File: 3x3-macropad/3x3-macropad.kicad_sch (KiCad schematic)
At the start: 38 parts, among them SW1 SW_Push, SW2 RotaryEncoder_Switch, U1 ATmega32U4-A, Y1 16MHz

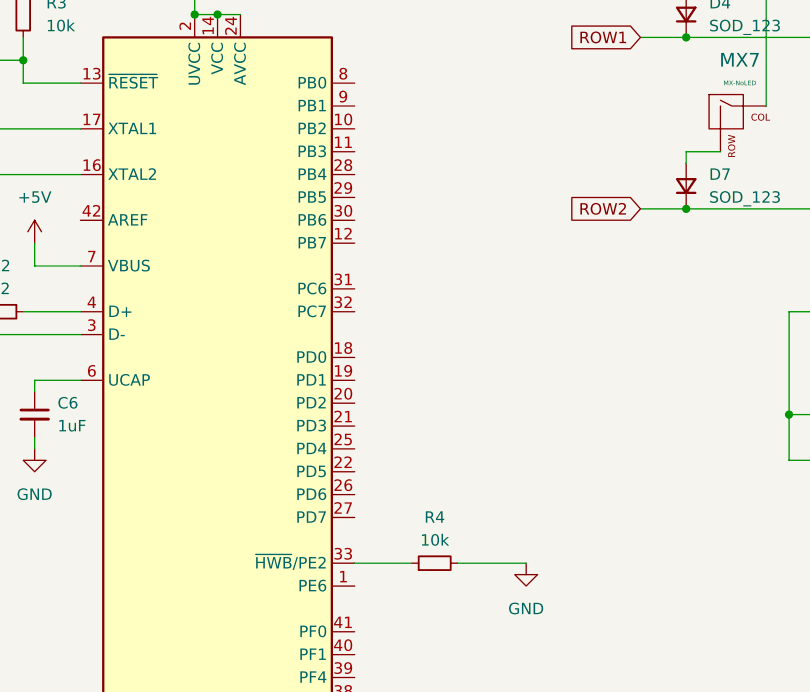
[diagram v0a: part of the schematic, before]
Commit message: first attempt routing 3x3
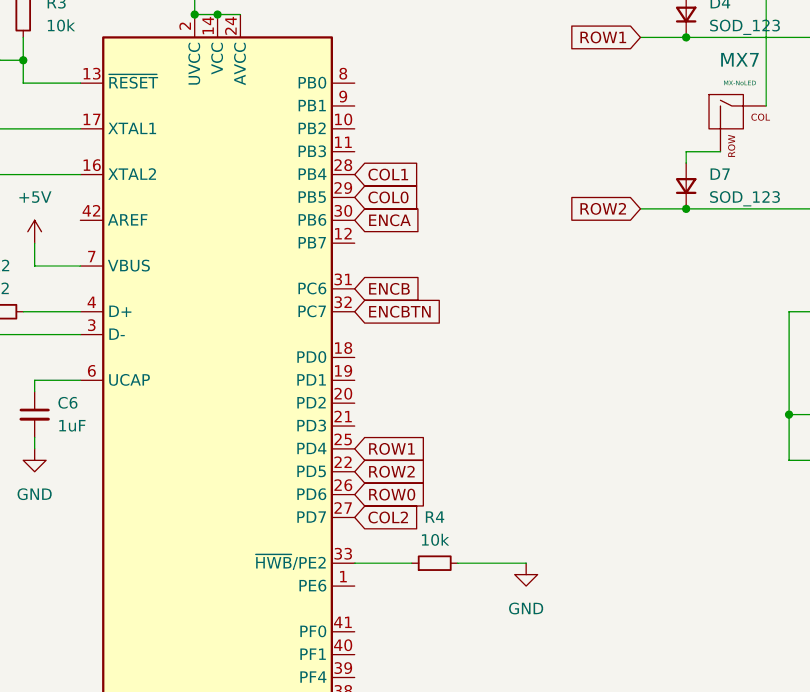
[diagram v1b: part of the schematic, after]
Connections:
- net COL0: now also U1.29 (PB5)
- net COL1: now also U1.28 (PB4)
- net COL2: now also U1.27 (PD7)
- net ENCA: now also U1.30 (PB6)
- net ENCB: now also U1.31 (PC6)
- net ENCBTN: now also U1.32 (PC7)
- net ROW0: now also U1.26 (PD6)
- net ROW1: now also U1.25 (PD4)
- net ROW2: now also U1.22 (PD5)
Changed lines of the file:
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@@
+    )
+  )
+  (global_label "ROW0" (shape input) (at 151.13 114.3 0) (fields_autoplaced)
+    (effects (font (size 1.27 1.27)) (justify left))
+    (property "Intersheetrefs" "${INTERSHEET_REFS}" (at 159.2972 114.3 0)
+      (effects (font (size 1.27 1.27)) (justify left) hide)
     )
   )
@@
     (effects (font (size 1.27 1.27)) (justify left))
     (property "Intersheetrefs" "${INTERSHEET_REFS}" (at 227.33 16.3861 90)
+      (effects (font (size 1.27 1.27)) (justify left) hide)
+    )
+  )
+  (global_label "COL1" (shape input) (at 151.13 78.74 0) (fields_autoplaced)
+    (effects (font (size 1.27 1.27)) (justify left))
+    (property "Intersheetrefs" "${INTERSHEET_REFS}" (at 158.8739 78.74 0)
+      (effects (font (size 1.27 1.27)) (justify left) hide)
+    )
+  )
+  (global_label "ENCBTN" (shape input) (at 151.13 93.98 0) (fields_autoplaced)
+    (effects (font (size 1.27 1.27)) (justify left))
+    (property "Intersheetrefs" "${INTERSHEET_REFS}" (at 161.3534 93.98 0)
+      (effects (font (size 1.27 1.27)) (justify left) hide)
+    )
+  )
+  (global_label "COL2" (shape input) (at 151.13 116.84 0) (fields_autoplaced)
+    (effects (font (size 1.27 1.27)) (justify left))
+    (property "Intersheetrefs" "${INTERSHEET_REFS}" (at 158.8739 116.84 0)
+      (effects (font (size 1.27 1.27)) (justify left) hide)
+    )
+  )
+  (global_label "COL0" (shape input) (at 151.13 81.28 0) (fields_autoplaced)
+    (effects (font (size 1.27 1.27)) (justify left))
+    (property "Intersheetrefs" "${INTERSHEET_REFS}" (at 158.8739 81.28 0)
+      (effects (font (size 1.27 1.27)) (justify left) hide)
+    )
+  )
+  (global_label "ENCA" (shape input) (at 151.13 83.82 0) (fields_autoplaced)
+    (effects (font (size 1.27 1.27)) (justify left))
+    (property "Intersheetrefs" "${INTERSHEET_REFS}" (at 158.8739 83.82 0)
       (effects (font (size 1.27 1.27)) (justify left) hide)
     )
@@
     (property "Intersheetrefs" "${INTERSHEET_REFS}" (at 212.09 128.3939 90)
       (effects (font (size 1.27 1.27)) (justify right) hide)
+    )
+  )
+  (global_label "ROW2" (shape input) (at 151.13 111.76 0) (fields_autoplaced)
+    (effects (font (size 1.27 1.27)) (justify left))
+    (property "Intersheetrefs" "${INTERSHEET_REFS}" (at 159.2972 111.76 0)
+      (effects (font (size 1.27 1.27)) (justify left) hide)
     )
   )
@@
     (effects (font (size 1.27 1.27)) (justify left))
     (property "Intersheetrefs" "${INTERSHEET_REFS}" (at 196.85 16.3861 90)
+      (effects (font (size 1.27 1.27)) (justify left) hide)
+    )
+  )
+  (global_label "ENCB" (shape input) (at 151.13 91.44 0) (fields_autoplaced)
+    (effects (font (size 1.27 1.27)) (justify left))
+    (property "Intersheetrefs" "${INTERSHEET_REFS}" (at 159.0553 91.44 0)
       (effects (font (size 1.27 1.27)) (justify left) hide)
     )
@@
     )
   )
+  (global_label "ROW1" (shape input) (at 151.13 109.22 0) (fields_autoplaced)
+    (effects (font (size 1.27 1.27)) (justify left))
+    (property "Intersheetrefs" "${INTERSHEET_REFS}" (at 159.2972 109.22 0)
+      (effects (font (size 1.27 1.27)) (justify left) hide)
+    )
+  )
